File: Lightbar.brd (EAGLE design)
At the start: 100 x 12 mm, 20 parts, among them IC1 PAM2863ECR, IC2 PAM2863ECR

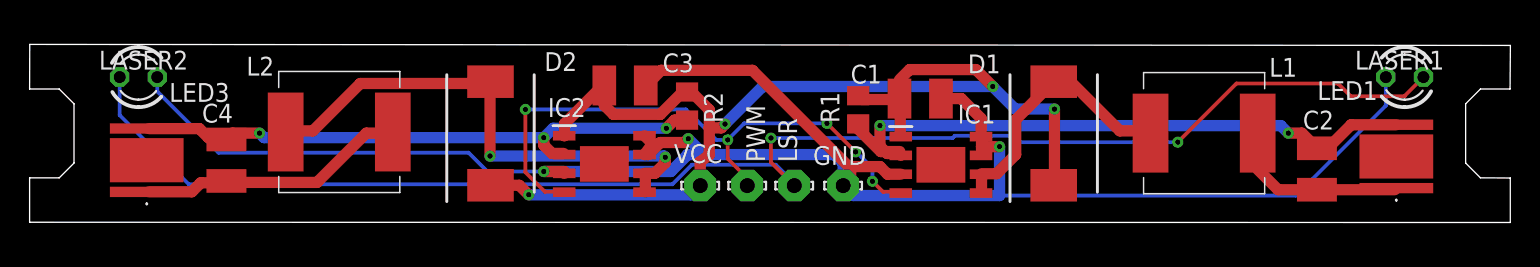
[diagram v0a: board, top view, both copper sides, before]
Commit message: Sensor Board Update
I also forgot what I updated here :((
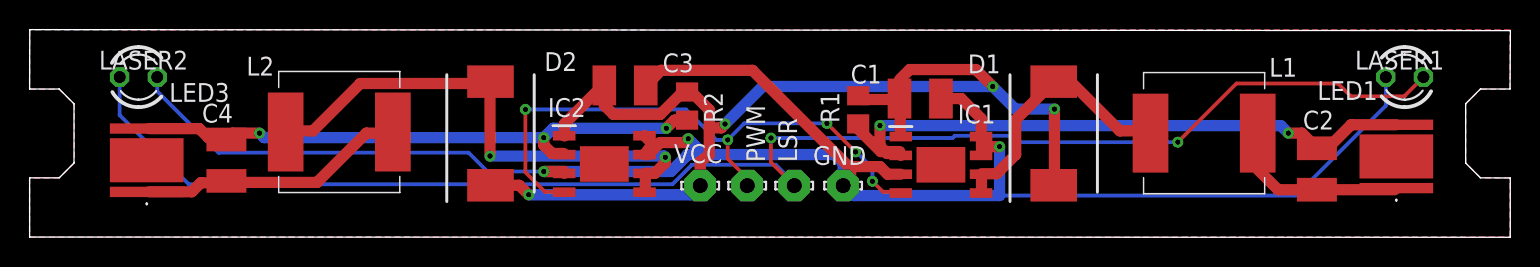
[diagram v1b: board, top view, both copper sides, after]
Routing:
- added copper zone on layer 1, net GND
- added copper zone on layer 16, net GND
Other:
- board size 100 x 12 mm -> 100 x 14 mm
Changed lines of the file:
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@@
 <board>
 <plain>
-<wire x1="0" y1="0" x2="100.0148" y2="-0.0162" width="0" layer="20"/>
-<wire x1="100.0148" y1="-0.0162" x2="100.0162" y2="2.9896" width="0" layer="20"/>
+<wire x1="0" y1="-1" x2="100.0148" y2="-1.0162" width="0" layer="20"/>
+<wire x1="100.0148" y1="-1.0162" x2="100.0162" y2="2.9896" width="0" layer="20"/>
 <wire x1="100.0162" y1="2.9896" x2="98" y2="3" width="0" layer="20"/>
 <wire x1="98" y1="3" x2="97" y2="4" width="0" layer="20"/>
@@
 <wire x1="97" y1="8" x2="98" y2="9" width="0" layer="20"/>
 <wire x1="98" y1="9" x2="100" y2="9" width="0" layer="20"/>
-<wire x1="100" y1="9" x2="100.023" y2="11.944" width="0" layer="20"/>
-<wire x1="100.023" y1="11.944" x2="0.0098" y2="12.0126" width="0" layer="20"/>
-<wire x1="0.0098" y1="12.0126" x2="0" y2="9" width="0" layer="20"/>
+<wire x1="100" y1="9" x2="100.023" y2="12.944" width="0" layer="20"/>
+<wire x1="100.023" y1="12.944" x2="0.0098" y2="13.0126" width="0" layer="20"/>
+<wire x1="0.0098" y1="13.0126" x2="0" y2="9" width="0" layer="20"/>
 <wire x1="0" y1="9" x2="2" y2="9" width="0" layer="20"/>
 <wire x1="2" y1="9" x2="3" y2="8" width="0" layer="20"/>
@@
 <wire x1="3" y1="4" x2="2" y2="3" width="0" layer="20"/>
 <wire x1="2" y1="3" x2="0" y2="3" width="0" layer="20"/>
-<wire x1="0" y1="3" x2="0" y2="0" width="0" layer="20"/>
+<wire x1="0" y1="3" x2="0" y2="-1" width="0" layer="20"/>
 </plain>
 <attributes>
@@
 <wire x1="54.951" y1="2.4765" x2="55.459" y2="2.9845" width="0.762" layer="1"/>
 <wire x1="55.459" y1="2.9845" x2="55.459" y2="3.6322" width="0.762" layer="1"/>
+<polygon width="0.2" layer="1" spacing="0.2" isolate="0.2">
+<vertex x="0" y="13"/>
+<vertex x="0" y="9"/>
+<vertex x="2" y="9"/>
+<vertex x="3" y="8"/>
+<vertex x="3" y="4"/>
+<vertex x="2" y="3"/>
+<vertex x="0" y="3"/>
+<vertex x="0" y="-1"/>
+<vertex x="100" y="-1"/>
+<vertex x="100" y="3"/>
+<vertex x="98" y="3"/>
+<vertex x="97" y="4"/>
+<vertex x="97" y="8"/>
+<vertex x="98" y="9"/>
+<vertex x="100" y="9"/>
+<vertex x="100" y="13"/>
+</polygon>
+<polygon width="0.2" layer="16" spacing="0.2" isolate="0.2">
+<vertex x="0" y="13"/>
+<vertex x="0" y="9"/>
+<vertex x="2" y="9"/>
+<vertex x="3" y="8"/>
+<vertex x="3" y="4"/>
+<vertex x="2" y="3"/>
+<vertex x="0" y="3"/>
+<vertex x="0" y="-1"/>
+<vertex x="100" y="-1"/>
+<vertex x="100" y="3"/>
+<vertex x="98" y="3"/>
+<vertex x="97" y="4"/>
+<vertex x="97" y="8"/>
+<vertex x="98" y="9"/>
+<vertex x="100" y="9"/>
+<vertex x="100" y="13"/>
+</polygon>
 </signal>
 <signal name="N$1">
